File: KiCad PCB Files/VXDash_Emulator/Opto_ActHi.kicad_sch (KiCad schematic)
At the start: 3 parts

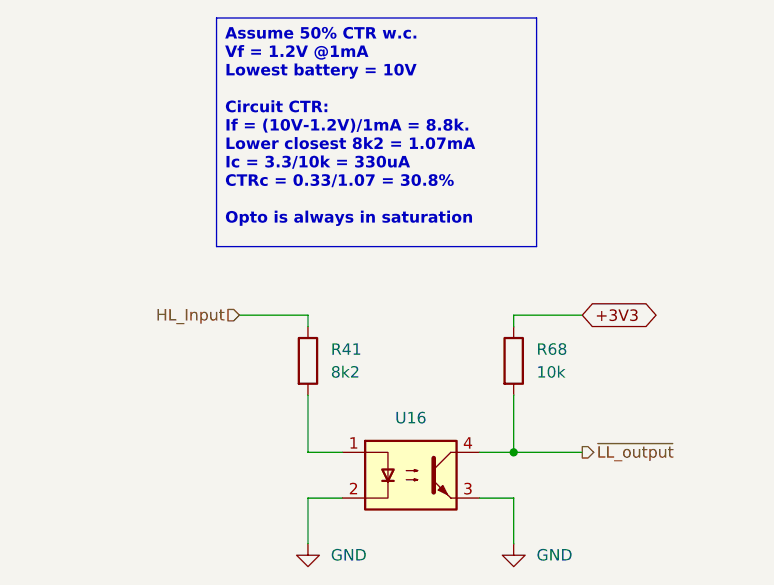
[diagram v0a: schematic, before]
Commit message: Emulator board refinements
- Is there stupid with the Active Hi Optos so that the logic is not inverted ?
- Added N-Mosfet activatable resistors. Stupidly simple ? Better MOSFET recommendation ?
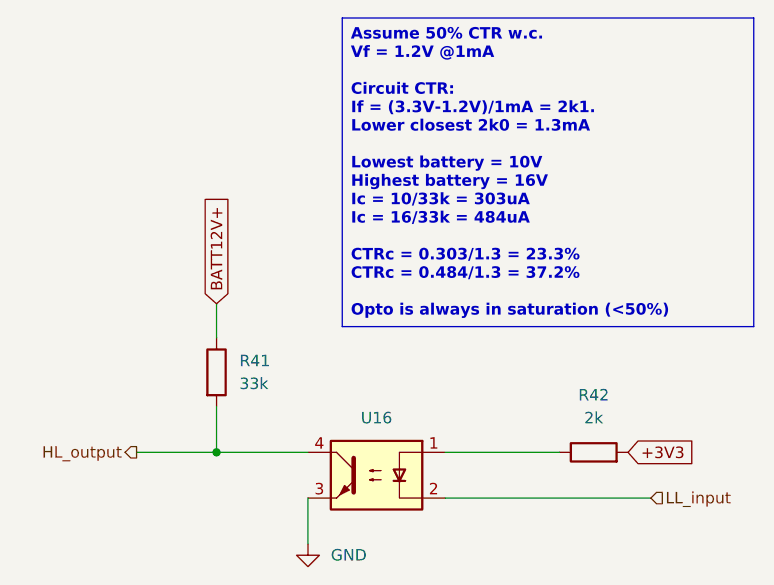
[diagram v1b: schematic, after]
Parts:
- R41: value 8k2 -> 33k
- R42: renamed from R68; value 10k -> 2k
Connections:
- net +3V3: now also R42.2; no longer R42.1
- net GND: no longer U16.2
- net at U16.1: now also R42.1; no longer R41.2
- net HL_Input renamed BATT12V+
- net ~{LL_output} renamed HL_output
- net HL_output: now also R41.2; no longer R42.2
- new net LL_input: U16.2
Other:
- moved on the sheet: R41, R42, U16
